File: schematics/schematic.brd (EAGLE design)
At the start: 140 x 100 mm, 58 parts, among them IC1 74HC365, T1 BC547, X5 PN61729-S

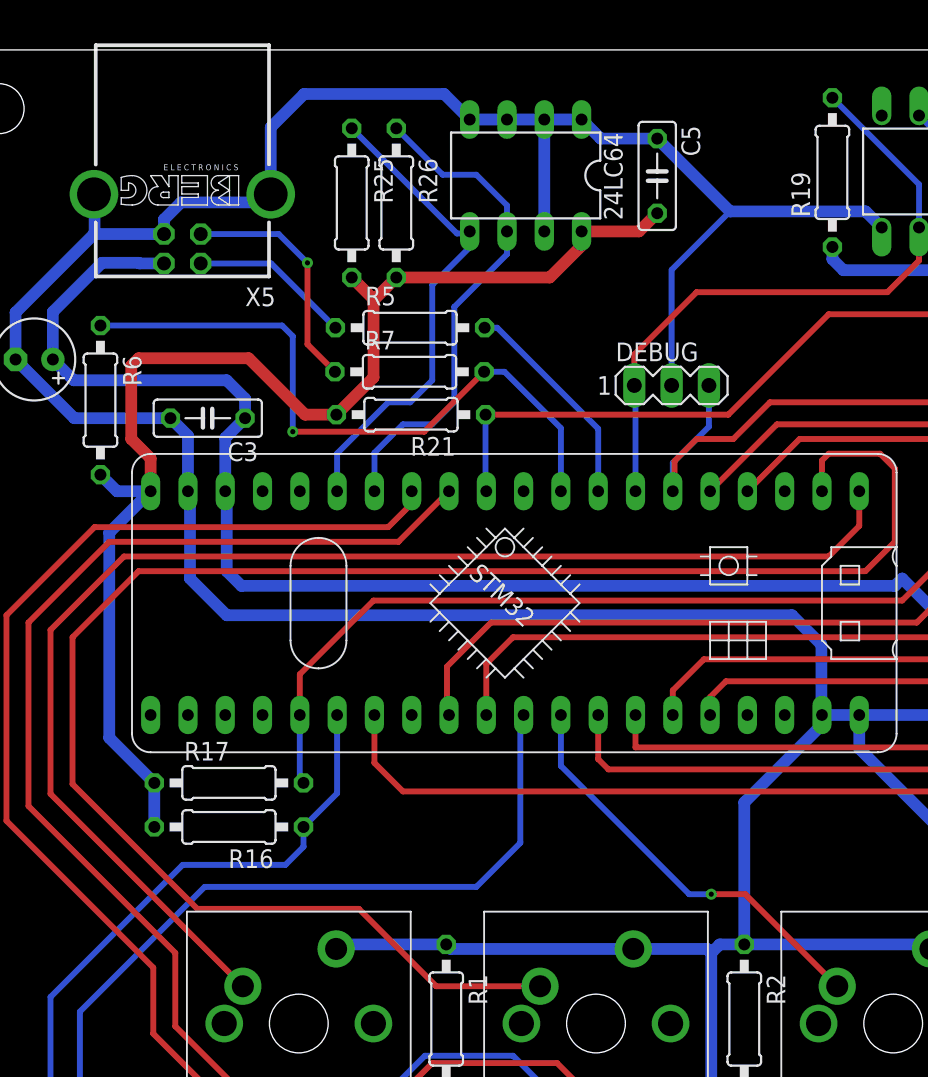
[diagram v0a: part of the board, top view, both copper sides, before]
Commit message: fixed some schematic errors
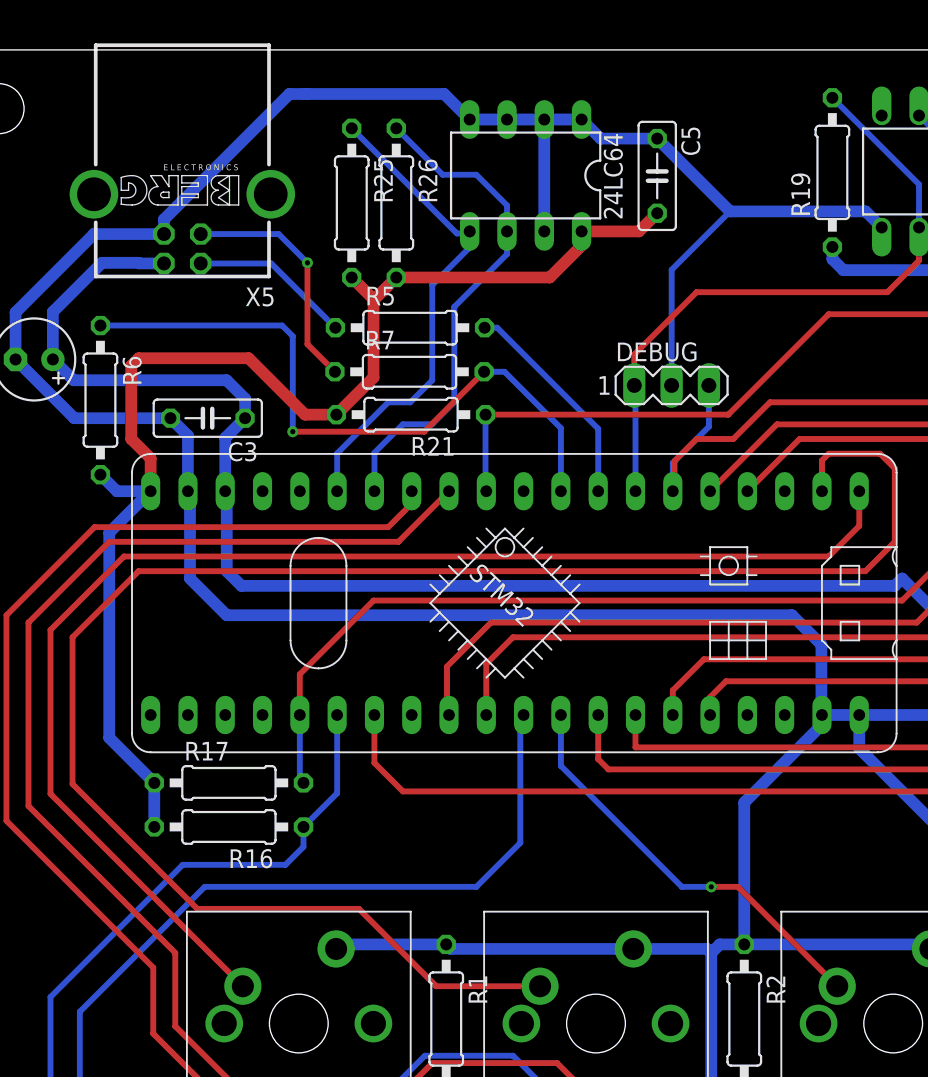
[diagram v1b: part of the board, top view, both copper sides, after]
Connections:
- net GND: no longer X5.S1, X5.S2
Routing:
- net GND: track 664.4 -> 659.1 mm
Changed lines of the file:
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@@
 </layers>
 <board>
-<fusionsync huburn="a.cGVyc29uYWw6dWUyOTRlZjhj" projecturn="a.cGVyc29uYWw6dWUyOTRlZjhjIzIwMTkwMTA1MTY4NDA4MjU2" f3durn="urn:adsk.wipprod:dm.lineage:Lq9hDvX_Sd6aCeZeqRCZkA" pcbguid="abaad317-76b8-409a-97c7-e120a538e6ae" lastpulledtime="" lastsyncedchangeguid="" latestrevisionid="7825f32e-bdc2-458f-9405-eec37679b984" lastsyncedrevisionid="7825f32e-bdc2-458f-9405-eec37679b984" lastboardhashguid="e4f4e491-0abb-39a3-c2ac-01114c3d0e76" lastpushedtime="2021-11-08T23:55:36Z" linktopcb3d="true"/>
+<fusionsync huburn="a.cGVyc29uYWw6dWUyOTRlZjhj" projecturn="a.cGVyc29uYWw6dWUyOTRlZjhjIzIwMTkwMTA1MTY4NDA4MjU2" f3durn="urn:adsk.wipprod:dm.lineage:Lq9hDvX_Sd6aCeZeqRCZkA" pcbguid="" lastpulledtime="" lastsyncedchangeguid="" latestrevisionid="7825f32e-bdc2-458f-9405-eec37679b984" lastsyncedrevisionid="7825f32e-bdc2-458f-9405-eec37679b984" lastboardhashguid="e4f4e491-0abb-39a3-c2ac-01114c3d0e76" lastpushedtime="2021-11-08T23:55:36Z" linktopcb3d="true"/>
 <plain>
 <wire x1="0" y1="0" x2="140" y2="0" width="0" layer="20"/>
@@
 <contactref element="R4" pad="1"/>
 <contactref element="X5" pad="4"/>
-<contactref element="X5" pad="S1"/>
-<contactref element="X5" pad="S2"/>
 <contactref element="M_OUT1" pad="P2"/>
 <contactref element="M_OUT2" pad="P2"/>
@@
 <wire x1="82" y1="54.705" x2="82" y2="54.63" width="0.4" layer="16"/>
 <wire x1="82" y1="54.63" x2="81.95" y2="54.58" width="0.4" layer="16"/>
-<wire x1="24.77" y1="97" x2="34.31" y2="97" width="0.8" layer="16"/>
+<wire x1="24.77" y1="97" x2="25" y2="97" width="0.8" layer="16"/>
+<wire x1="25" y1="97" x2="34.31" y2="97" width="0.8" layer="16"/>
 <wire x1="49.8" y1="77.15" x2="49.8" y2="85.02" width="0.4" layer="16"/>
 <wire x1="49.8" y1="85.02" x2="53.78" y2="89" width="0.4" layer="16"/>
 <wire x1="15.23" y1="87.46" x2="15.23" y2="88.46" width="0.8" layer="16"/>
-<wire x1="16.385" y1="89.615" x2="15.23" y2="88.46" width="0.8" layer="16"/>
-<wire x1="16.385" y1="89.615" x2="21.945" y2="89.615" width="0.8" layer="16"/>
-<wire x1="21.945" y1="89.615" x2="22.5" y2="90.17" width="0.8" layer="16"/>
-<wire x1="22.5" y1="90.17" x2="22.5" y2="94.73" width="0.8" layer="16"/>
-<wire x1="22.5" y1="94.73" x2="24.77" y2="97" width="0.8" layer="16"/>
+<wire x1="16.385" y1="89.615" x2="16.135" y2="89.365" width="0.8" layer="16"/>
+<wire x1="16.135" y1="89.365" x2="15.23" y2="88.46" width="0.8" layer="16"/>
 <wire x1="87.45" y1="42.3" x2="84.91" y2="44.84" width="0.4" layer="16"/>
 <wire x1="84.91" y1="44.84" x2="79.83" y2="44.84" width="0.4" layer="16"/>
@@
 <wire x1="43.67" y1="95.26" x2="44.97" y2="93.96" width="0.8" layer="16"/>
 <wire x1="41.13" y1="87.64" x2="41.13" y2="95.26" width="0.8" layer="16"/>
-<wire x1="10.5" y1="90.13" x2="10.46" y2="90.17" width="0.8" layer="16"/>
-<wire x1="10.5" y1="87.5" x2="10.5" y2="90.13" width="0.8" layer="16"/>
 <wire x1="54.75" y1="39.08" x2="67.12305" y2="39.08" width="0.8" layer="16"/>
 <wire x1="67.12305" y1="39.08" x2="67.43" y2="38.77305" width="0.8" layer="16"/>
 <wire x1="104.56" y1="49.42" x2="100.5" y2="45.36" width="0.8" layer="16"/>
 <wire x1="100.5" y1="45.36" x2="100.5" y2="34" width="0.8" layer="16"/>
+<wire x1="16.385" y1="89.615" x2="23.77" y2="97" width="0.8" layer="16"/>
+<wire x1="23.77" y1="97" x2="24.77" y2="97" width="0.8" layer="16"/>
 </signal>
 <signal name="PB12">
@@
 <contactref element="STM32F103" pad="P$29"/>
 <wire x1="42.26" y1="54.705" x2="42.26" y2="51.24" width="0.4" layer="16"/>
-<wire x1="51" y1="42.5" x2="52.5" y2="42.5" width="0.4" layer="16"/>
-<wire x1="42.26" y1="51.24" x2="51" y2="42.5" width="0.4" layer="16"/>
-<via x="52.5" y="42.5" extent="1-16" drill="0.35"/>
-<wire x1="61.08" y1="36.23305" x2="54.81305" y2="42.5" width="0.4" layer="1"/>
-<wire x1="52.5" y1="42.5" x2="54.81305" y2="42.5" width="0.4" layer="1"/>
+<wire x1="50.5" y1="43" x2="52.5" y2="43" width="0.4" layer="16"/>
+<wire x1="42.26" y1="51.24" x2="50.5" y2="43" width="0.4" layer="16"/>
+<via x="52.5" y="43" extent="1-16" drill="0.35"/>
+<wire x1="61.08" y1="36.23305" x2="54.31305" y2="43" width="0.4" layer="1"/>
+<wire x1="52.5" y1="43" x2="54.31305" y2="43" width="0.4" layer="1"/>
 </signal>
 <signal name="N$4">
